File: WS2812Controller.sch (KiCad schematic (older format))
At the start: 16 parts, among them J1 USB_B_Micro, J2 Conn_01x05_Male, J3 Conn_01x03, SW1 SW_Reset, SW2 SW_GPIO0, U1 AMS1117-3.3, U2 ESP-12F

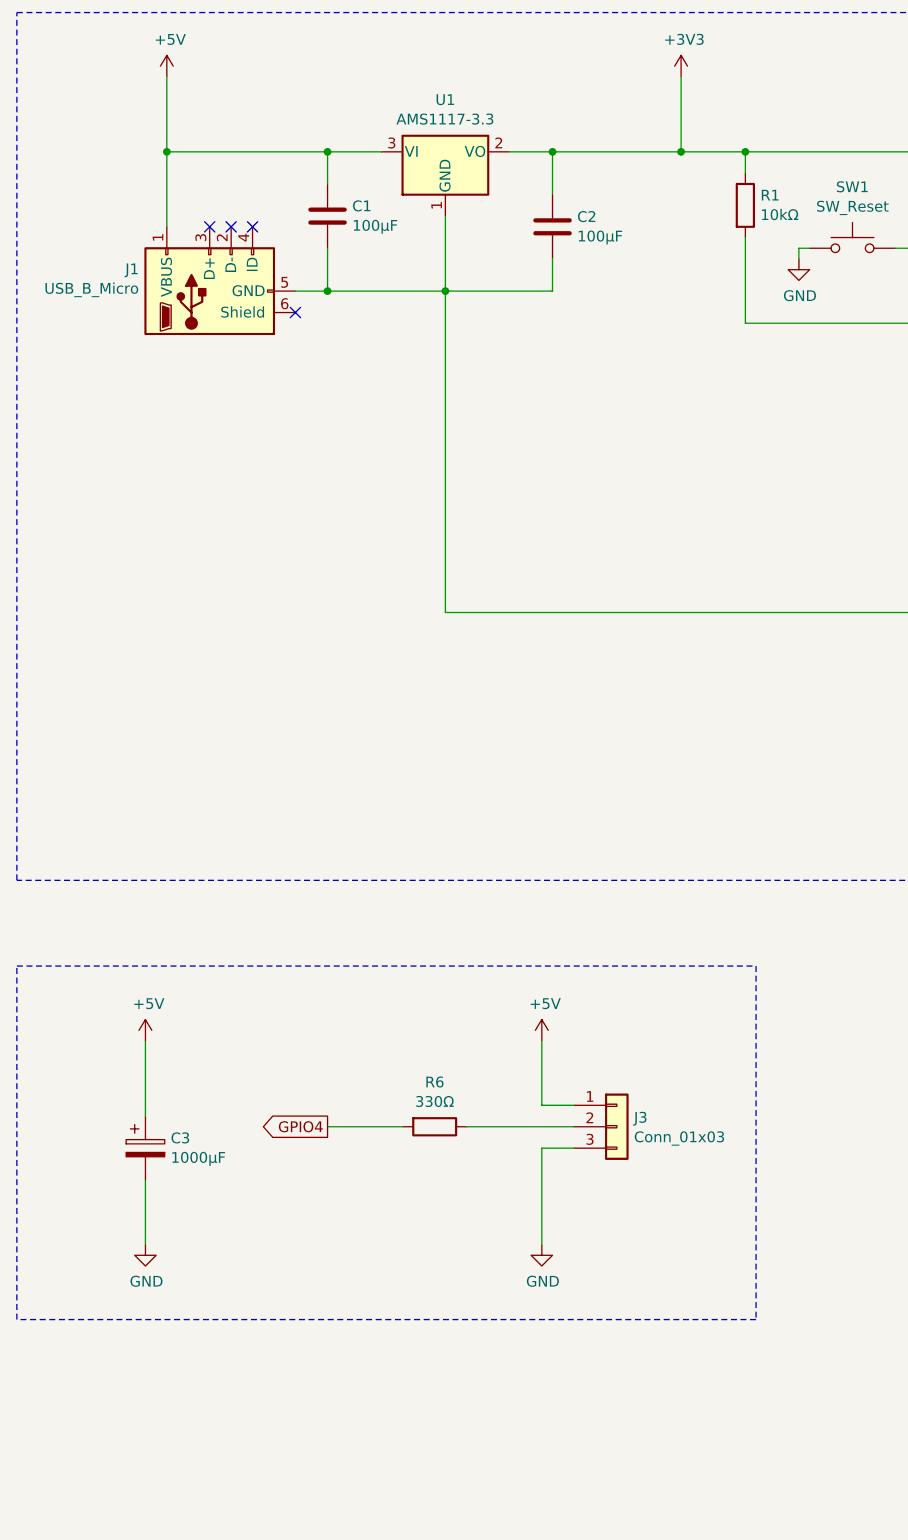
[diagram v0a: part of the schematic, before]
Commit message: New layout
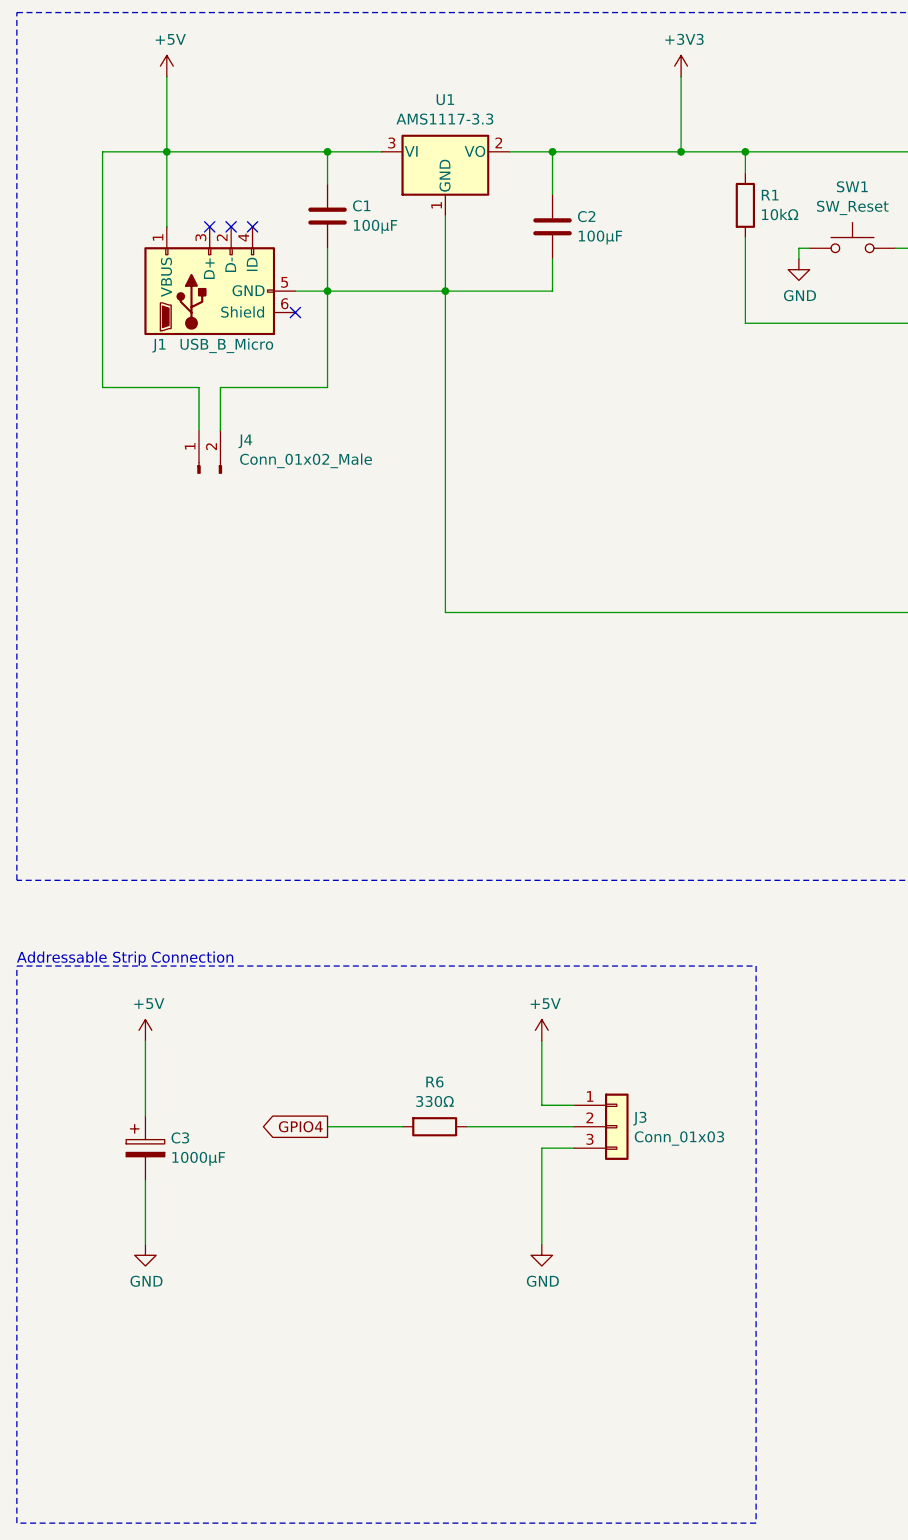
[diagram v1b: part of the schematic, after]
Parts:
- added J4: Conn_01x02_Male, TerminalBlock:TerminalBlock_bornier-2_P5.08mm, symbol Connector:Conn_01x02_Male
- J3: footprint halibs:SolderPads3 -> TerminalBlock_Phoenix:TerminalBlock_Phoenix_MPT-0,5-3-2.54_1x03_P2.54mm_Horizontal
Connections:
- net +5V: now also J4.1 (Pin_1)
- net GND: now also J4.2 (Pin_2)
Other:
- note added: "Addressable Strip Connection"
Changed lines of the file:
@@
 U 1 1 5C938411
 P 1600 1900
-F 0 "J1" V 1702 2230 50  0000 L CNN
-F 1 "USB_B_Micro" V 1611 2230 50  0000 L CNN
+F 0 "J1" V 1350 2100 50  0000 L CNN
+F 1 "USB_B_Micro" V 1350 1600 50  0000 L CNN
 F 2 "Connector_USB:USB_Micro-B_Molex_47346-0001" H 1750 1850 50  0001 C CNN
 F 3 "~" H 1750 1850 50  0001 C CNN
@@
 F 0 "J3" H 3580 5842 50  0000 L CNN
 F 1 "Conn_01x03" H 3580 5751 50  0000 L CNN
-F 2 "halibs:SolderPads3" H 3500 5800 50  0001 C CNN
+F 2 "TerminalBlock_Phoenix:TerminalBlock_Phoenix_MPT-0,5-3-2.54_1x03_P2.54mm_Horizontal" H 3500 5800 50  0001 C CNN
 F 3 "~" H 3500 5800 50  0001 C CNN
 	1    3500 5800
@@
 	700  5050 4150 5050
 Wire Notes Line
-	4150 5050 4150 6700
-Wire Notes Line
-	4150 6700 700  6700
-Wire Notes Line
-	700  6700 700  5050
+	4150 5050 4150 7650
+Wire Notes Line
+	4150 7650 700  7650
+Wire Notes Line
+	700  7650 700  5050
 Wire Wire Line
 	7450 1250 9850 1250
@@
 Wire Wire Line
 	4950 2050 4100 2050
+Text Notes 700  5050 0    50   ~ 0
+Addressable Strip Connection
+$Comp
+L Connector:Conn_01x02_Male J4
+U 1 1 6096D0BC
+P 1550 2750
+F 0 "J4" V 1704 2562 50  0000 R CNN
+F 1 "Conn_01x02_Male" V 1613 2562 50  0000 R CNN
+F 2 "TerminalBlock:TerminalBlock_bornier-2_P5.08mm" H 1550 2750 50  0001 C CNN
+F 3 "~" H 1550 2750 50  0001 C CNN
+	1    1550 2750
+	0    -1   -1   0
+$EndComp
+Wire Wire Line
+	1550 2550 1550 2350
+Wire Wire Line
+	1550 2350 1100 2350
+Wire Wire Line
+	1100 2350 1100 1250
+Wire Wire Line
+	1100 1250 1400 1250
+Wire Wire Line
+	1650 2550 1650 2350
+Wire Wire Line
+	1650 2350 2150 2350
+Wire Wire Line
+	2150 2350 2150 1900
 $EndSCHEMATC
